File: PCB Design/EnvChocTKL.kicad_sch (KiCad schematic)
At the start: 190 parts, among them J1 Type-c-31-m-14

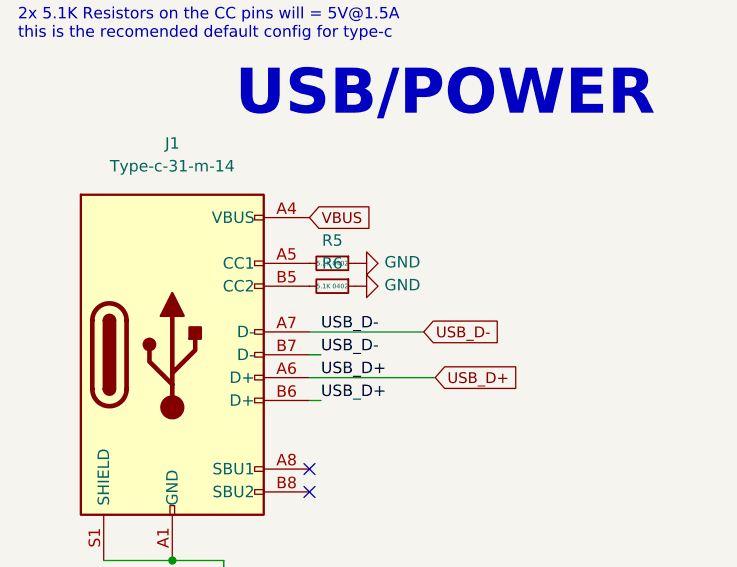
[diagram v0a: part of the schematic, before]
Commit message: generated updated gerber
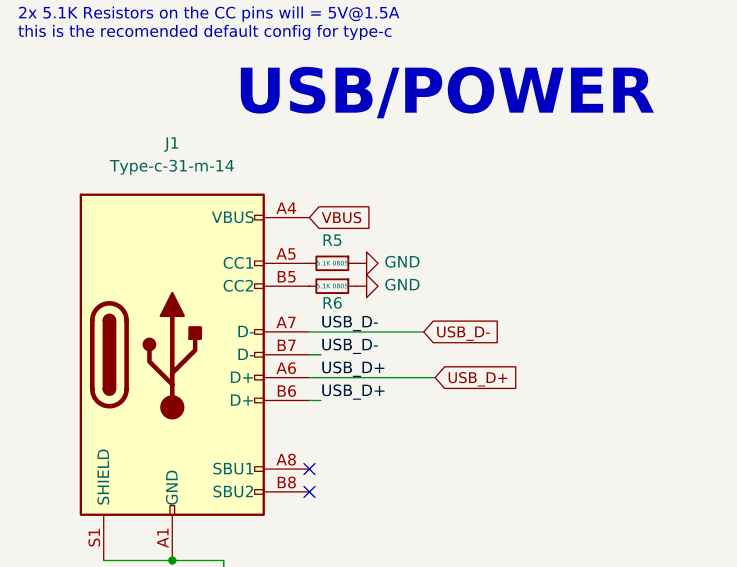
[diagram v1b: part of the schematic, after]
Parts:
- R5, R6: value 5.1K 0402 -> 5.1K 0805; footprint Resistor_SMD:R_0402_1005Metric -> Resistor_SMD:R_0805_2012Metric
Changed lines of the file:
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@@
   (symbol (lib_id "Device:R_Small") (at 50.165 46.355 270) (unit 1)
     (in_bom yes) (on_board yes)
-    (property "Reference" "R6" (id 0) (at 50.165 43.815 90))
-    (property "Value" "5.1K 0402" (id 1) (at 50.165 46.355 90)
+    (property "Reference" "R6" (id 0) (at 50.165 48.26 90))
+    (property "Value" "5.1K 0805" (id 1) (at 50.165 46.355 90)
       (effects (font (size 0.508 0.508)))
     )
-    (property "Footprint" "Resistor_SMD:R_0402_1005Metric" (id 2) (at 50.165 46.355 0)
+    (property "Footprint" "Resistor_SMD:R_0805_2012Metric" (id 2) (at 50.165 46.355 0)
       (effects (font (size 1.27 1.27)) hide)
     )
@@
     (in_bom yes) (on_board yes)
     (property "Reference" "R5" (id 0) (at 50.165 41.275 90))
-    (property "Value" "5.1K 0402" (id 1) (at 50.165 43.815 90)
+    (property "Value" "5.1K 0805" (id 1) (at 50.165 43.815 90)
       (effects (font (size 0.508 0.508)))
     )
-    (property "Footprint" "Resistor_SMD:R_0402_1005Metric" (id 2) (at 50.165 43.815 0)
+    (property "Footprint" "Resistor_SMD:R_0805_2012Metric" (id 2) (at 50.165 43.815 0)
       (effects (font (size 1.27 1.27)) hide)
     )
@@
     )
     (path "/00000000-0000-0000-0000-00006093a5b0"
-      (reference "R5") (unit 1) (value "5.1K 0402") (footprint "Resistor_SMD:R_0402_1005Metric")
+      (reference "R5") (unit 1) (value "5.1K 0805") (footprint "Resistor_SMD:R_0805_2012Metric")
     )
     (path "/00000000-0000-0000-0000-0000609385d4"
-      (reference "R6") (unit 1) (value "5.1K 0402") (footprint "Resistor_SMD:R_0402_1005Metric")
+      (reference "R6") (unit 1) (value "5.1K 0805") (footprint "Resistor_SMD:R_0805_2012Metric")
     )
     (path "/6be092fb-5a07-4210-ab9f-d96af1d79bdc"
